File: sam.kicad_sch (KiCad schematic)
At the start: 56 parts, among them IC1 HYB4116, IC15 MC6883, IC16 74LS244N, IC2 HYB4116, IC3 HYB4116, IC31 74LS02N, IC33 74LS138N, IC4 HYB4116, IC5 HYB4116, IC6 HYB4116, IC7 HYB4116, IC8 HYB4116

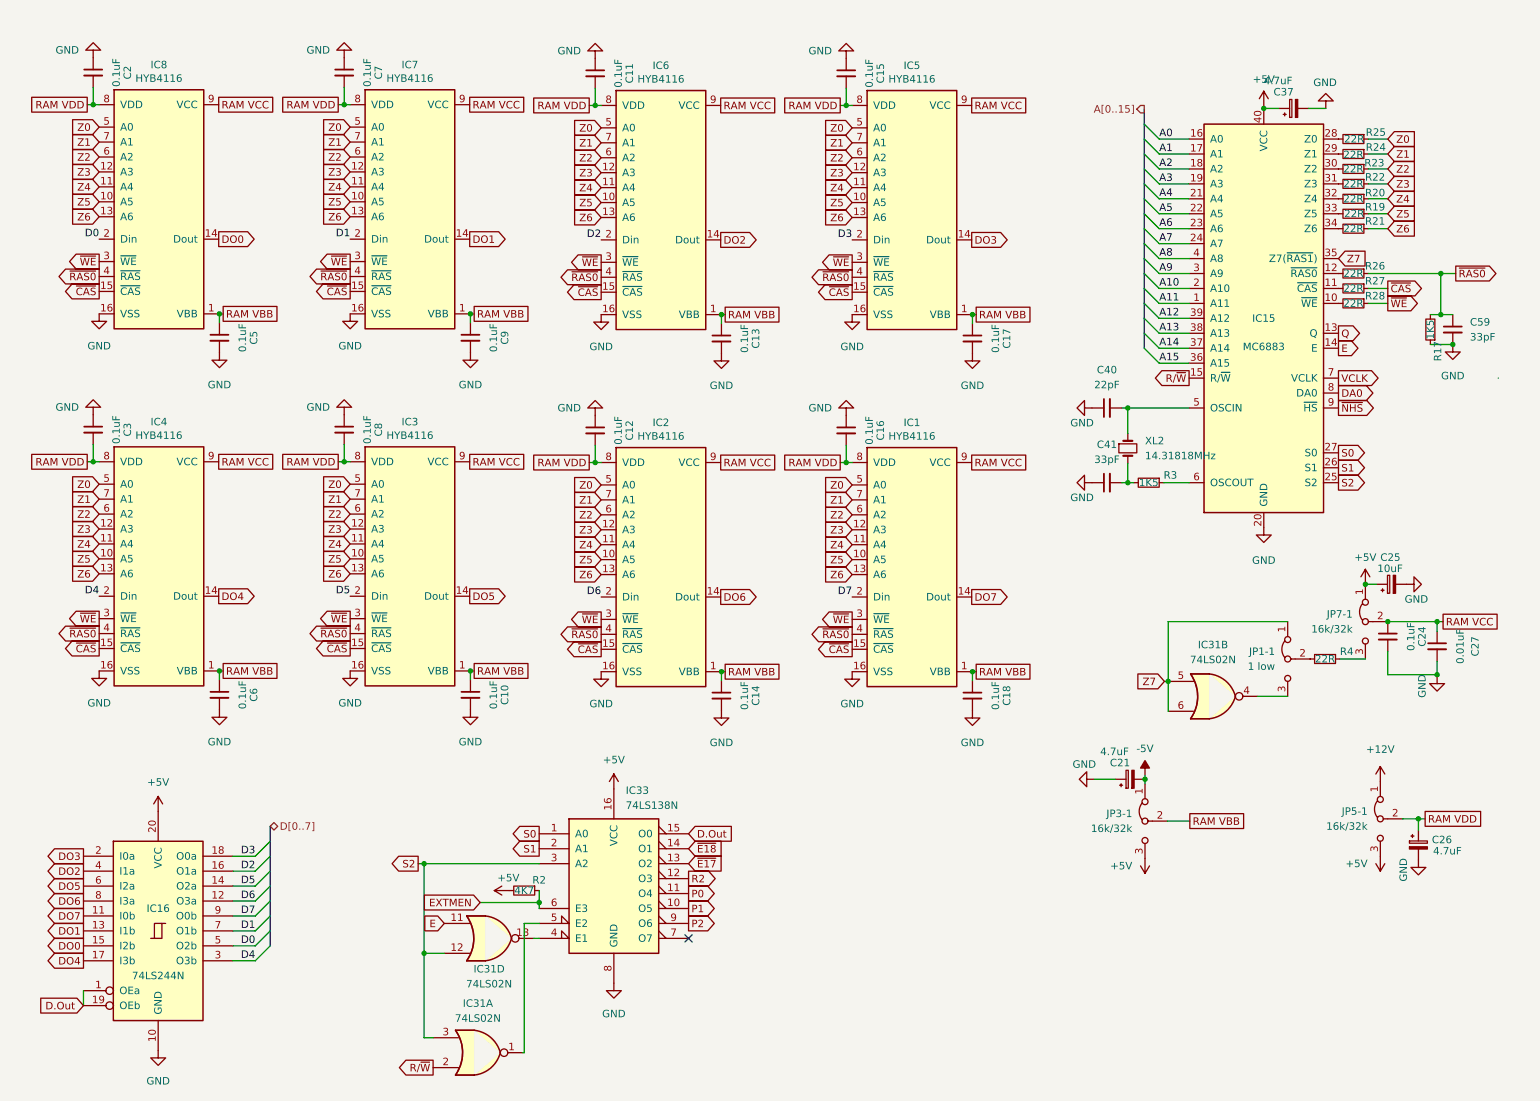
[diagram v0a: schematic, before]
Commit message: work on memory sub system
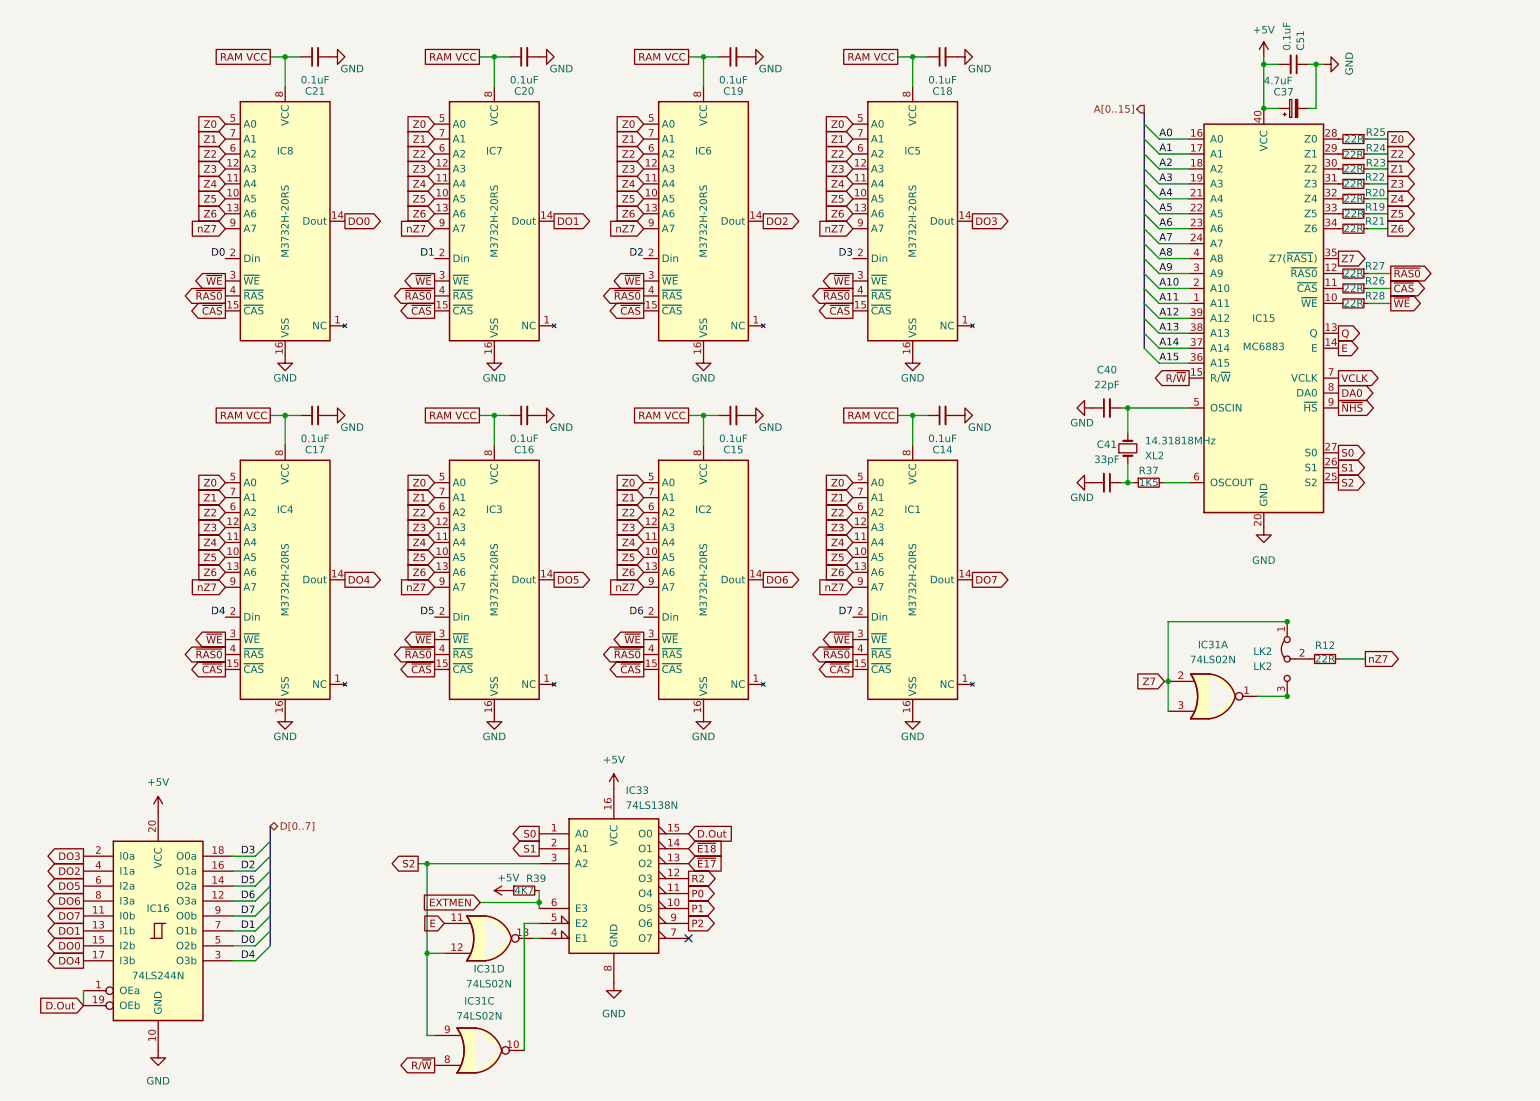
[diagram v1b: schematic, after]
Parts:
- removed C10, C11, C12, C13, C14, C2, C24, C3, C5, C6, C7, C8, C9: 0.1uF, Capacitor_THT:C_Disc_D4.3mm_W1.9mm_P5.00mm, symbol Device:C_Small
- removed C21, C26: 4.7uF, Capacitor_THT:CP_Radial_D5.0mm_P2.50mm, symbol Device:C_Polarized_Small
- removed C25: 10uF, Capacitor_THT:CP_Radial_D5.0mm_P2.50mm, symbol Device:C_Polarized_Small
- removed C27: 0.01uF, Capacitor_THT:C_Disc_D4.3mm_W1.9mm_P5.00mm, symbol Device:C_Small
- removed C59: 33pF, Capacitor_THT:C_Disc_D4.3mm_W1.9mm_P5.00mm, symbol Device:C_Small
- removed IC2, IC3, IC4, IC5, IC6, IC7, IC8: HYB4116, Package_DIP:DIP-16_W7.62mm, symbol Memory_RAM_Siemens:HYB4116
- removed JP1-1: 1 low, Connector_PinHeader_2.54mm:PinHeader_1x03_P2.54mm_Vertical, symbol Jumper:Jumper_3_Bridged12
- removed JP3-1, JP5-1, JP7-1: 16k/32k, Connector_PinHeader_2.54mm:PinHeader_1x03_P2.54mm_Vertical, symbol Jumper:Jumper_3_Bridged12
- removed R17: 1K5, Resistor_THT:R_Axial_DIN0309_L9.0mm_D3.2mm_P12.70mm_Horizontal, symbol Device:R_Small
- added C16, C19, C20, C21, C51: 0.1uF, Capacitor_THT:C_Disc_D4.3mm_W1.9mm_P5.00mm, symbol Device:C_Small
- added IC2, IC3, IC4, IC5, IC6, IC7, IC8: M3732H-20RS, Package_DIP:DIP-16_W7.62mm, symbol vdg:MSM3732
- added LK2: LK2, Connector_PinHeader_2.54mm:PinHeader_1x03_P2.54mm_Vertical, symbol Jumper:Jumper_3_Bridged12
- C37: footprint Capacitor_THT:CP_Radial_D5.0mm_P2.50mm -> Capacitor_THT:CP_Radial_Tantal_D5.5mm_P5.00mm
- C40: footprint Capacitor_THT:C_Disc_D4.3mm_W1.9mm_P5.00mm -> Dragon:C_Radial_Special
- C41: footprint Capacitor_THT:C_Disc_D4.3mm_W1.9mm_P5.00mm -> Capacitor_THT:C_Disc_D3.0mm_W1.6mm_P2.50mm
- IC1: value HYB4116 -> M3732H-20RS; symbol Memory_RAM_Siemens:HYB4116 -> vdg:MSM3732
- R12: renamed from R4; footprint Resistor_THT:R_Axial_DIN0309_L9.0mm_D3.2mm_P12.70mm_Horizontal -> Dragon:R_Axial_DIN0309_L9.0mm_D2.5mm_P12.70mm_Horizontal
- R19, R20, R21, R22, R23, R24, R25, R28: footprint Resistor_THT:R_Axial_DIN0309_L9.0mm_D3.2mm_P12.70mm_Horizontal -> Dragon:R_Axial_DIN0309_L9.0mm_D2.5mm_P12.70mm_Horizontal
- R26: renamed from R27; footprint Resistor_THT:R_Axial_DIN0309_L9.0mm_D3.2mm_P12.70mm_Horizontal -> Dragon:R_Axial_DIN0309_L9.0mm_D2.5mm_P12.70mm_Horizontal
- R27: renamed from R26; footprint Resistor_THT:R_Axial_DIN0309_L9.0mm_D3.2mm_P12.70mm_Horizontal -> Dragon:R_Axial_DIN0309_L9.0mm_D2.5mm_P12.70mm_Horizontal
- R37: renamed from R3; footprint Resistor_THT:R_Axial_DIN0309_L9.0mm_D3.2mm_P12.70mm_Horizontal -> Dragon:R_Axial_DIN0309_L9.0mm_D2.5mm_P12.70mm_Horizontal
- R39: renamed from R2; footprint Resistor_THT:R_Axial_DIN0309_L9.0mm_D3.2mm_P12.70mm_Horizontal -> Dragon:R_Axial_DIN0309_L9.0mm_D2.5mm_P12.70mm_Horizontal
- renumbered C16 to C14
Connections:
- net +5V: now also R39.1, C51.2; no longer R39.2
- net D0: now also IC8.2 (Din)
- net D1: now also IC7.2 (Din)
- net D2: now also IC6.2 (Din)
- net D3: now also IC5.2 (Din)
- net D4: now also IC4.2 (Din)
- net D5: now also IC3.2 (Din)
- net D6: now also IC2.2 (Din)
- net DO0: now also IC8.14 (Dout)
- net DO1: now also IC7.14 (Dout)
- net DO2: now also IC6.14 (Dout)
- net DO3: now also IC5.14 (Dout)
- net DO4: now also IC4.14 (Dout)
- net DO5: now also IC3.14 (Dout)
- net DO6: now also IC2.14 (Dout)
- net EXTMEN: now also R39.2; no longer R39.1
- net GND: now also C14.2, C15.2, C41.2, C16.2, C19.2, C20.2, C21.2, C51.1, IC2.16 (VSS), IC3.16 (VSS), IC4.16 (VSS), IC5.16 (VSS), IC6.16 (VSS), IC7.16 (VSS), IC8.16 (VSS); no longer C14.1, C15.1, C41.1
- net RAM VCC: now also C14.1, C15.1, C17.1, C18.1, IC1.8 (VCC), C16.1, C19.1, C20.1, C21.1, IC2.8 (VCC), IC3.8 (VCC), IC4.8 (VCC), IC5.8 (VCC), IC6.8 (VCC), IC7.8 (VCC), IC8.8 (VCC); no longer IC1.9 (VCC)
- net R/~{W}: now also IC31.8; no longer IC31.2
- net S2: now also IC31.9; no longer IC31.3
- net Z0: now also IC2.5 (A0), IC3.5 (A0), IC4.5 (A0), IC5.5 (A0), IC6.5 (A0), IC7.5 (A0), IC8.5 (A0)
- net Z1: now also R23.1, IC2.7 (A1), IC3.7 (A1), IC4.7 (A1), IC5.7 (A1), IC6.7 (A1), IC7.7 (A1), IC8.7 (A1); no longer R24.1
- net Z2: now also R24.1, IC2.6 (A2), IC3.6 (A2), IC4.6 (A2), IC5.6 (A2), IC6.6 (A2), IC7.6 (A2), IC8.6 (A2); no longer R23.1
- net Z3: now also IC2.12 (A3), IC3.12 (A3), IC4.12 (A3), IC5.12 (A3), IC6.12 (A3), IC7.12 (A3), IC8.12 (A3)
- net Z4: now also IC2.11 (A4), IC3.11 (A4), IC4.11 (A4), IC5.11 (A4), IC6.11 (A4), IC7.11 (A4), IC8.11 (A4)
- net Z5: now also IC2.10 (A5), IC3.10 (A5), IC4.10 (A5), IC5.10 (A5), IC6.10 (A5), IC7.10 (A5), IC8.10 (A5)
- net Z6: now also IC2.13 (A6), IC3.13 (A6), IC4.13 (A6), IC5.13 (A6), IC6.13 (A6), IC7.13 (A6), IC8.13 (A6)
- net Z7: now also IC31.2, IC31.3, LK2.1 (A); no longer IC31.5, IC31.6
- net ~{CAS}: now also IC2.15 (~{CAS}), IC3.15 (~{CAS}), IC4.15 (~{CAS}), IC5.15 (~{CAS}), IC6.15 (~{CAS}), IC7.15 (~{CAS}), IC8.15 (~{CAS})
- net ~{RAS0}: now also IC2.4 (~{RAS}), IC3.4 (~{RAS}), IC4.4 (~{RAS}), IC5.4 (~{RAS}), IC6.4 (~{RAS}), IC7.4 (~{RAS}), IC8.4 (~{RAS})
- net ~{WE}: now also IC2.3 (~{WE}), IC3.3 (~{WE}), IC4.3 (~{WE}), IC5.3 (~{WE}), IC6.3 (~{WE}), IC7.3 (~{WE}), IC8.3 (~{WE})
- net nZ7: now reaches R12.1
- net nZ7: now also IC1.9 (A7), IC2.9 (A7), IC3.9 (A7), IC4.9 (A7), IC5.9 (A7), IC6.9 (A7), IC7.9 (A7), IC8.9 (A7)
- net at C40.2, IC15.5 (OSCIN): now also XL2.2; no longer XL2.1
- net at R37.1: now also C41.1, XL2.1; no longer IC15.6 (OSCOUT)
- net at IC33.5 (E2): now also IC31.10; no longer IC31.1
- removed net RAM VBB: C17.1, C18.1, IC1.1 (VBB)
- removed net RAM VDD: C14.2, C15.2, IC1.8 (VDD)
- new net: IC15.6 (OSCOUT), R37.2
- new net: IC31.1, LK2.3 (B)
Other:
- moved on the sheet: C14, C41, R37, R39
